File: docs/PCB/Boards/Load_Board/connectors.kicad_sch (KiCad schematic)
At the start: 18 parts, among them J21 R_IN, J22 R_OUT, J23 SW_IN, J24 SW_OUT, J25 Divider_1, J26 Divider_2, J27 BZ_IN, J28 BZ_OUT, J29 LED_IN, J30 LED_OUT, J31 CRYSTAL_IN, J32 CRYSTAL_OUT, J33 T_1, J34 T_2, J35 L_IN, J36 L_OUT, J37 C_IN, J38 C_OUT

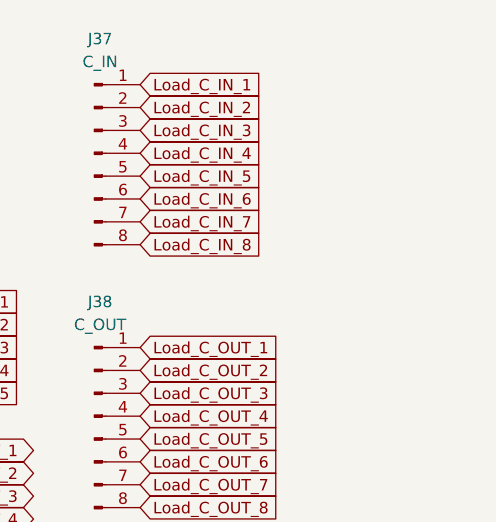
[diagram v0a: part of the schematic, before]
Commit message: Hardware docs updated.
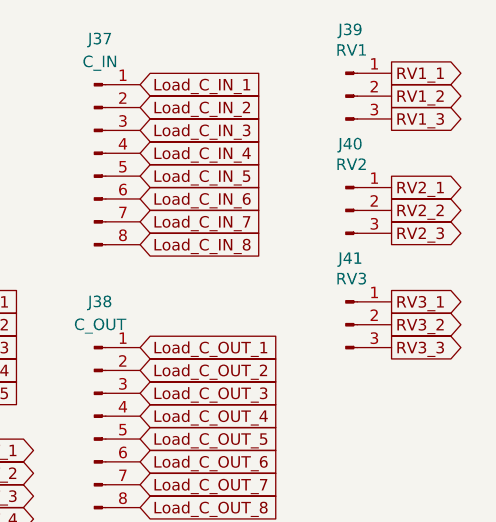
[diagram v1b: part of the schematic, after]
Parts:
- added J39: RV1, Connector_PinSocket_2.54mm:PinSocket_1x03_P2.54mm_Vertical, symbol Connector:Conn_01x03_Pin
- added J40: RV2, Connector_PinSocket_2.54mm:PinSocket_1x03_P2.54mm_Vertical, symbol Connector:Conn_01x03_Pin
- added J41: RV3, Connector_PinSocket_2.54mm:PinSocket_1x03_P2.54mm_Vertical, symbol Connector:Conn_01x03_Pin
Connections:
- new net RV1_1: J39.1 (Pin_1)
- new net RV1_2: J39.2 (Pin_2)
- new net RV1_3: J39.3 (Pin_3)
- new net RV2_1: J40.1 (Pin_1)
- new net RV2_2: J40.2 (Pin_2)
- new net RV2_3: J40.3 (Pin_3)
- new net RV3_1: J41.1 (Pin_1)
- new net RV3_2: J41.2 (Pin_2)
- new net RV3_3: J41.3 (Pin_3)
